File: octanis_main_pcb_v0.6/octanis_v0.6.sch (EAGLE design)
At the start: 106 parts, among them IC1 BME280, IC2 BNO055A, Q1 32.768kHz, Q2 32.768kHz, U1 TPS61232, U10 INA210, U11 INA210, U12 INA210, U13 RN2483, U2 DRV8836DSSR, U3 DRV8836DSSR, U4 MSP432, U5 SST25VF064C, U6 DRV8836DSSR, U7 DRV8836DSSR, U8 MAX6001SOT-23, U9 INA210

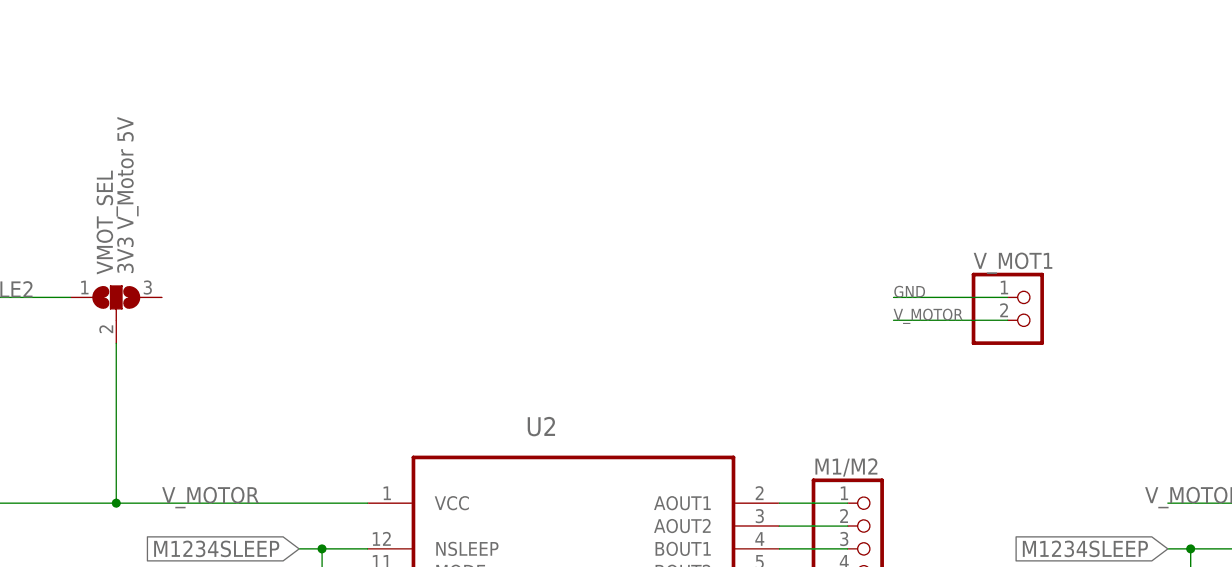
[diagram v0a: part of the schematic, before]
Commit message: DRC clean layout
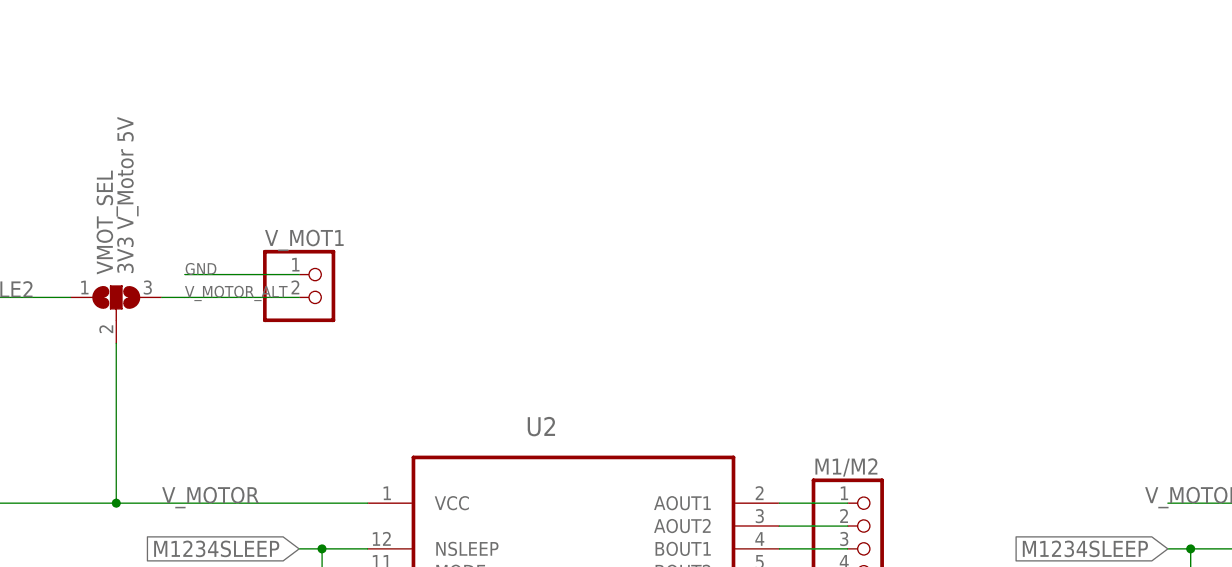
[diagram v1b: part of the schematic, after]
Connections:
- new net V_MOTOR_ALT: VMOT_SEL.3, V_MOT1.2
- net V_MOTOR: no longer V_MOT1.2
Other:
- moved on the sheet: V_MOT1
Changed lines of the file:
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@@
 <instance part="JP1" gate="A" x="193.04" y="297.18"/>
 <instance part="V_MOT2" gate="A" x="563.88" y="142.24"/>
-<instance part="V_MOT1" gate="A" x="314.96" y="129.54"/>
+<instance part="V_MOT1" gate="A" x="236.22" y="132.08"/>
 <instance part="X3" gate="G$1" x="144.78" y="490.22" rot="R90"/>
 <instance part="JP4" gate="A" x="226.06" y="434.34"/>
@@
 <segment>
 <pinref part="V_MOT1" gate="A" pin="1"/>
-<wire x1="312.42" y1="132.08" x2="299.72" y2="132.08" width="0.1524" layer="91"/>
-<label x="299.72" y="132.08" size="1.27" layer="95"/>
+<wire x1="233.68" y1="134.62" x2="220.98" y2="134.62" width="0.1524" layer="91"/>
+<label x="220.98" y="134.62" size="1.27" layer="95"/>
 </segment>
 <segment>
@@
 <label x="327.66" y="109.22" size="1.778" layer="95"/>
 </segment>
-<segment>
-<pinref part="V_MOT1" gate="A" pin="2"/>
-<wire x1="312.42" y1="129.54" x2="299.72" y2="129.54" width="0.1524" layer="91"/>
-<label x="299.72" y="129.54" size="1.27" layer="95"/>
-</segment>
 </net>
 <net name="N$2" class="0">
@@
 </segment>
 </net>
+<net name="V_MOTOR_ALT" class="3">
+<segment>
+<pinref part="V_MOT1" gate="A" pin="2"/>
+<wire x1="233.68" y1="132.08" x2="220.98" y2="132.08" width="0.1524" layer="91"/>
+<label x="220.98" y="132.08" size="1.27" layer="95"/>
+<pinref part="VMOT_SEL" gate="G$1" pin="3"/>
+<wire x1="220.98" y1="132.08" x2="218.44" y2="132.08" width="0.1524" layer="91"/>
+</segment>
+</net>
